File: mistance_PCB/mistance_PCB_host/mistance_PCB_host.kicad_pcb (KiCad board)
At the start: 2 copper layers, 90 x 90.5 mm, 88 parts, among them J3 GRPB052VWVN-RC, J4 OLED, J5 SMA-J-P-X-ST-TH1, Q1 Q_PMOS_DSG, Q2 UMH3N, U1 ESP32-WROOM-32E, U2 TPS61200DRC, U3 MCP73831-2-OT, U4 AMS1117-3.3, U5 CP2104, U6 TPS3839DBZ, U7 SX1278, U8 USBLC6-2P6, Y1 Crystal

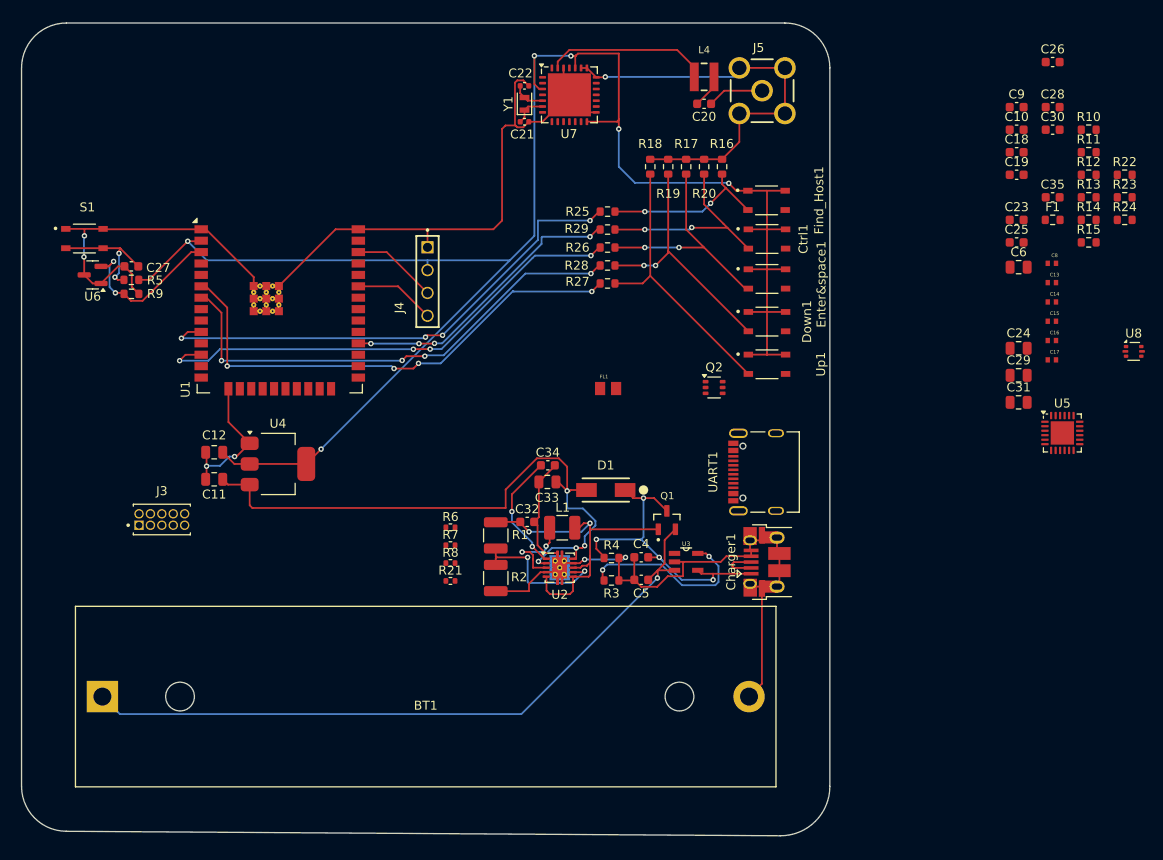
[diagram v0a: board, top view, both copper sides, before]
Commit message: PCB writing
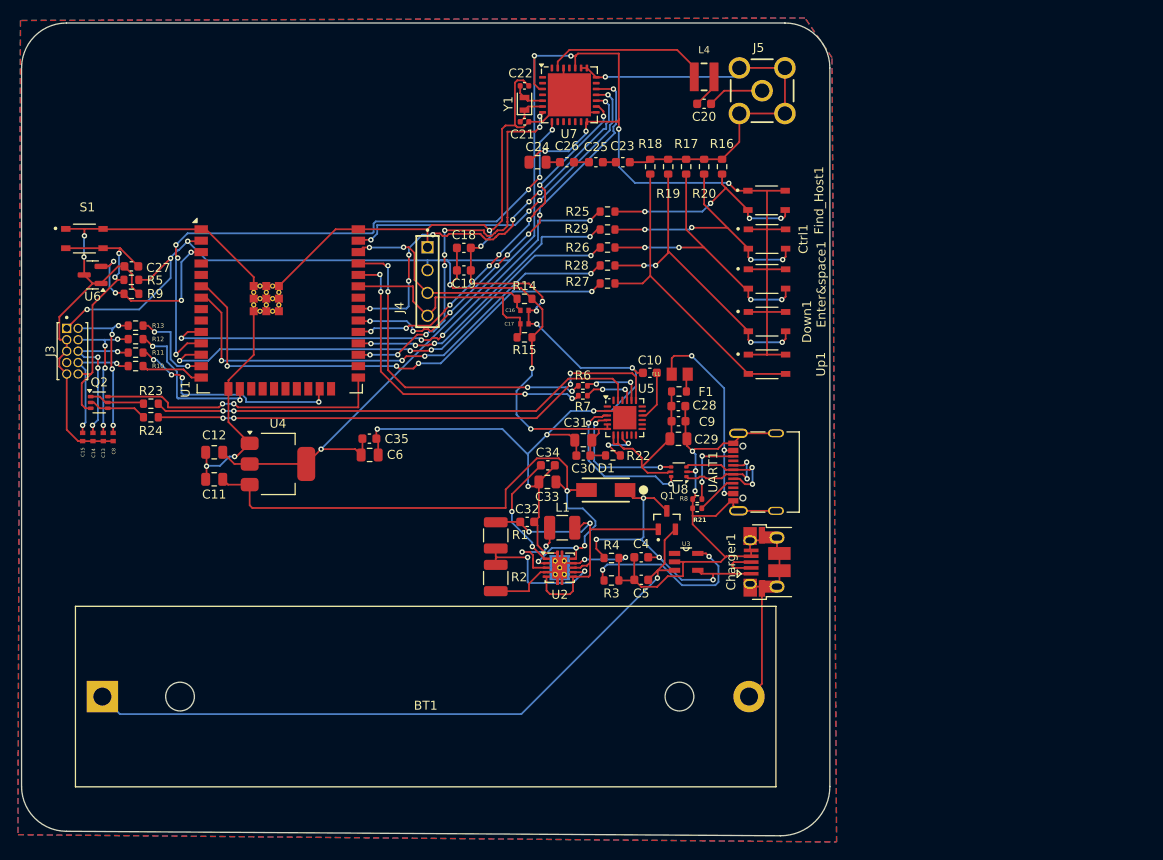
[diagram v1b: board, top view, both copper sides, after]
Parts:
- R21: value 22R -> 5.1K
- moved R23 110.8 mm to (29.4, 57.4)
- moved R24 110.6 mm to (29.4, 58.9)
- moved R10 109.3 mm to (27.7, 53.2), turned to 180 degrees
- moved C15 108.7 mm to (21.8, 61.1), turned to -90 degrees
- moved R11 108.4 mm to (27.7, 51.7), turned to 180 degrees
- moved C14 107.8 mm to (22.9, 61.1), turned to -90 degrees
- moved R12 107.7 mm to (27.7, 50.2), turned to 180 degrees
- moved R13 107.1 mm to (27.7, 48.7), turned to 180 degrees
- moved C13 107.0 mm to (24.1, 61.1), turned to -90 degrees
- moved C8 106.3 mm to (25.2, 61.1), turned to -90 degrees
- moved C35 80.7 mm to (53.7, 61.3)
- moved C6 75.2 mm to (53.8, 63.1)
- moved Q2 68.5 mm to (23.6, 57.2)
- moved R22 65.0 mm to (80.8, 63.1), turned to 180 degrees
- moved R15 63.7 mm to (71.0, 50.0)
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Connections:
- UART1 pad A1_B12: (no net) -> GND
- UART1 pad A4_B9: (no net) -> Net-(FL1-Pad2)
- UART1 pad B1_A12: (no net) -> GND
- UART1 pad B4_A9: (no net) -> Net-(FL1-Pad2)
- UART1 pad SH1: (no net) -> GND
- UART1 pad SH2: (no net) -> GND
- UART1 pad SH3: (no net) -> GND
- UART1 pad SH4: (no net) -> GND
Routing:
- net GND: track 242.2 -> 408.7 mm, vias 7 -> 20
- net 3.3V OUT: track 198.5 -> 279.0 mm, vias 6 -> 13
- net DIO0(IRQ): track 0.00 -> 66.7 mm, vias 0 -> 6
- net Net-(U5-~{RTS}): track 0.00 -> 58.8 mm, vias 0 -> 4
- net Net-(U5-~{DTR}): track 0.00 -> 55.1 mm, vias 0 -> 2
- net NSS(CS): track 0.00 -> 46.7 mm, vias 0 -> 8
- net MISO: track 0.00 -> 45.3 mm, vias 0 -> 8
- net RESET: track 0.00 -> 45.3 mm, vias 0 -> 8
- net SCK: track 0.00 -> 41.7 mm, vias 0 -> 8
- net MOSI: track 0.00 -> 39.2 mm, vias 0 -> 4
- net TX: track 0.00 -> 37.4 mm, vias 0 -> 4
- net RX: track 0.00 -> 36.7 mm, vias 0 -> 4
- net IO0: track 0.00 -> 32.4 mm, vias 0 -> 2
- net MTDO: track 0.00 -> 24.7 mm, vias 0 -> 4
- net Net-(FL1-Pad2): track 0.00 -> 23.0 mm, vias 0 -> 3
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- added copper zone on B.Cu, net GND
- added copper zone on F.Cu, net GND
